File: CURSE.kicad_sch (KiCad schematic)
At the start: 25 parts, among them J1 USB_C_Receptacle_USB2.0_14P, U1 RP2040, U2 NCP1117-3.3_SOT223, Y1 12 Mhz

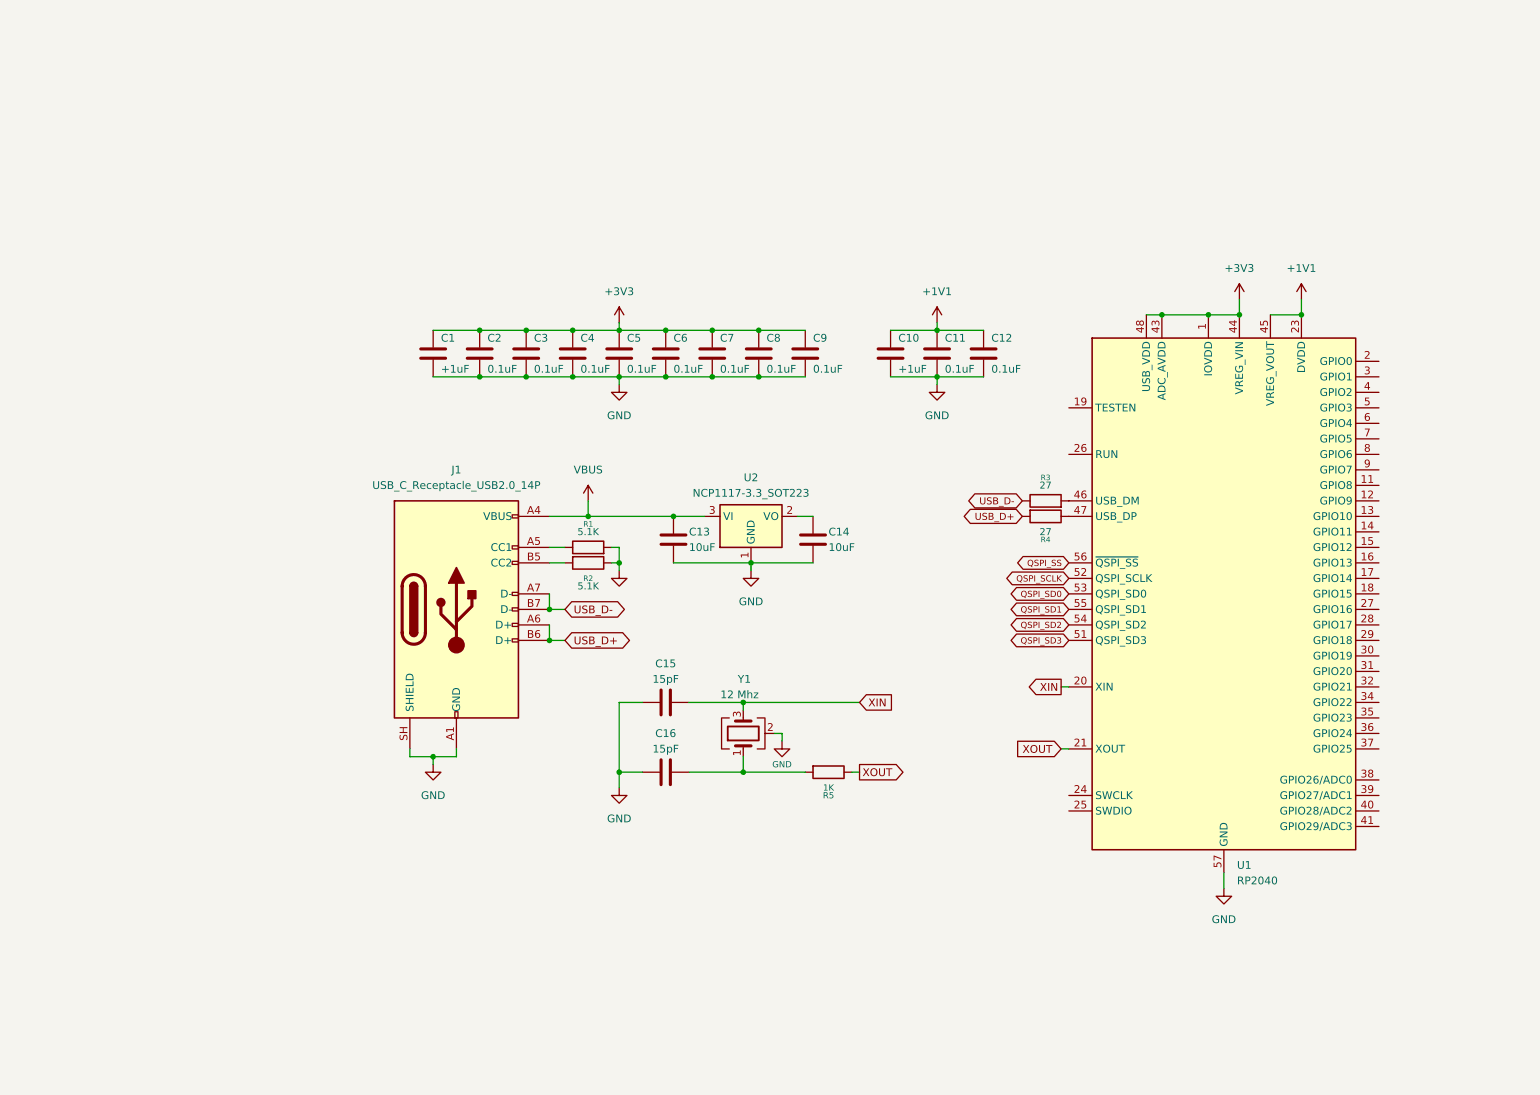
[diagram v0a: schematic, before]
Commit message: now going on with pcb!! check the devlog for what made
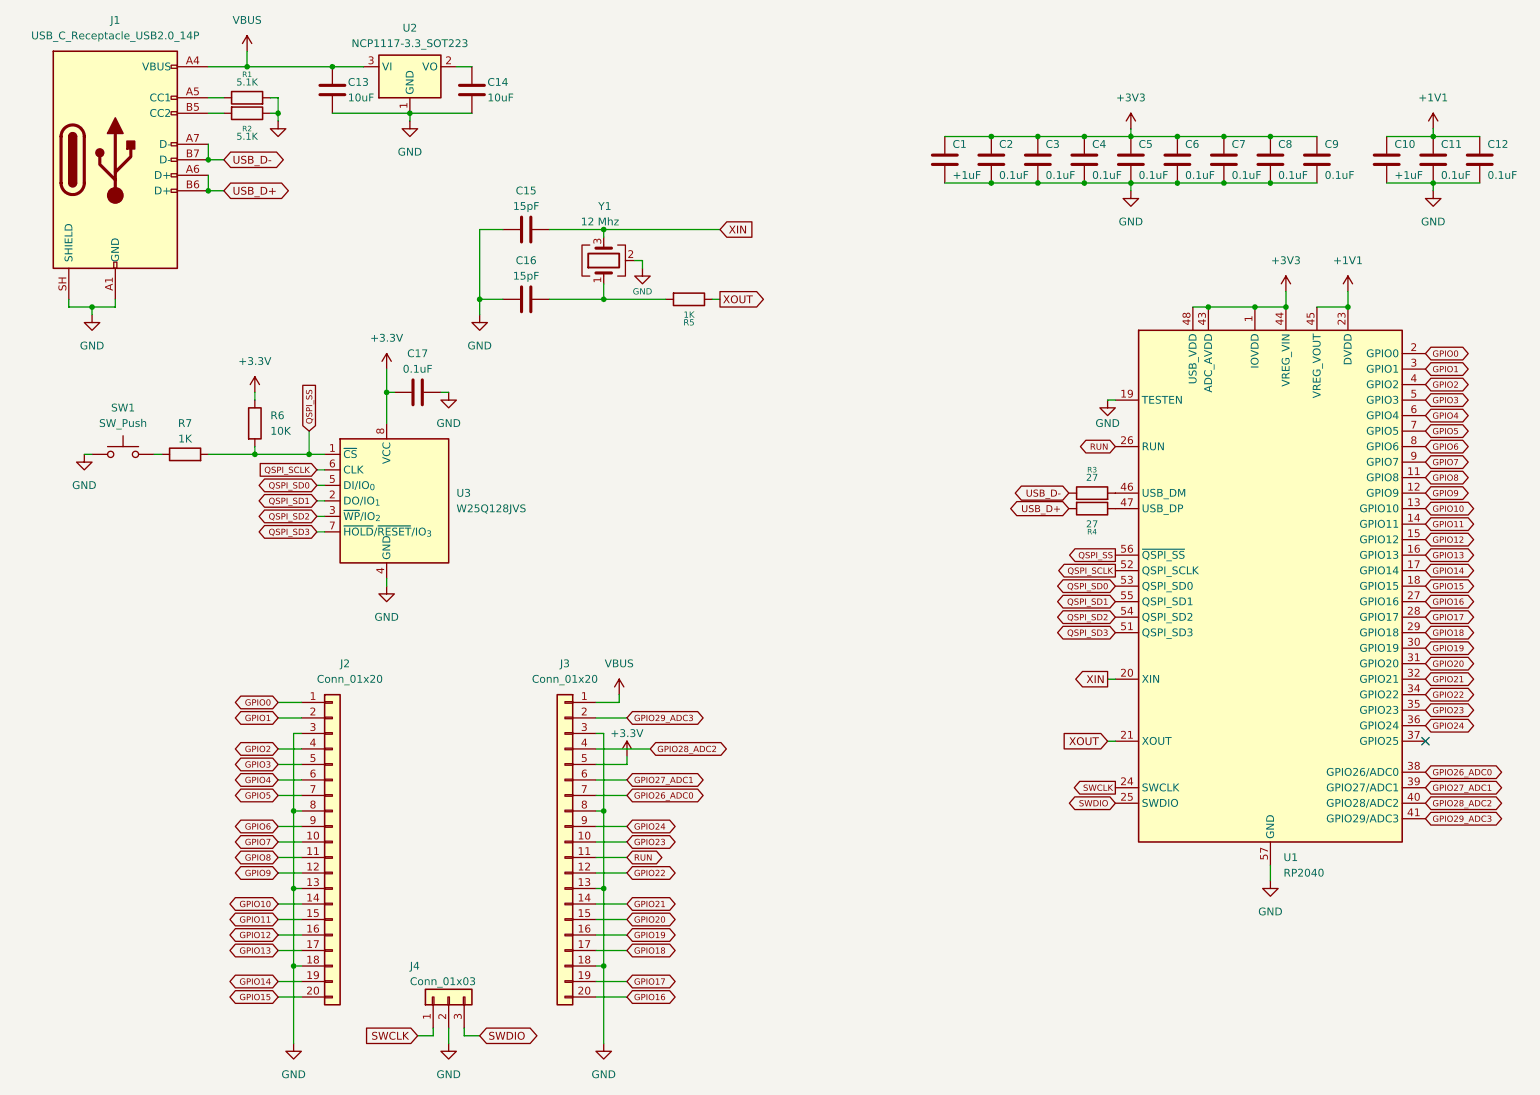
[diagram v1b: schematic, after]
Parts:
- added C17: 0.1uF, symbol Device:C
- added J2, J3: Conn_01x20, symbol Connector_Generic:Conn_01x20
- added J4: Conn_01x03, symbol Connector_Generic:Conn_01x03
- added R6: 10K, symbol Device:R
- added R7: 1K, symbol Device:R
- added SW1: SW_Push, symbol Switch:SW_Push
- added U3: W25Q128JVS, Package_SO:SOIC-8_5.3x5.3mm_P1.27mm, symbol Memory_Flash:W25Q128JVS
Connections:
- net GND: now also U1.19 (TESTEN), C17.2, J2.13 (Pin_13), J2.18 (Pin_18), J2.3 (Pin_3), J2.8 (Pin_8), J3.13 (Pin_13), J3.18 (Pin_18), J3.3 (Pin_3), J3.8 (Pin_8), J4.2 (Pin_2), SW1.1, U3.4 (GND)
- net QSPI_SCLK: now also U3.6 (CLK)
- net QSPI_SD0: now also U3.5 (DI/IO_{0})
- net QSPI_SD1: now also U3.2 (DO/IO_{1})
- net QSPI_SD2: now also U3.3 (~{WP}/IO_{2})
- net QSPI_SD3: now also U3.7 (~{HOLD}/~{RESET}/IO_{3})
- net QSPI_SS: now also R6.2, R7.2, U3.1 (~{CS})
- net VBUS: now also J3.1 (Pin_1)
- net GPIO8: now reaches U1.11 (GPIO8)
- net GPIO8: now also J2.11 (Pin_11)
- net GPIO9: now reaches U1.12 (GPIO9)
- net GPIO9: now also J2.12 (Pin_12)
- net GPIO10: now reaches U1.13 (GPIO10)
- net GPIO10: now also J2.14 (Pin_14)
- net GPIO11: now reaches U1.14 (GPIO11)
- net GPIO11: now also J2.15 (Pin_15)
- net GPIO12: now reaches U1.15 (GPIO12)
- net GPIO12: now also J2.16 (Pin_16)
- net GPIO13: now reaches U1.16 (GPIO13)
- net GPIO13: now also J2.17 (Pin_17)
- net GPIO14: now reaches U1.17 (GPIO14)
- net GPIO14: now also J2.19 (Pin_19)
- net GPIO15: now reaches U1.18 (GPIO15)
- net GPIO15: now also J2.20 (Pin_20)
- net GPIO0: now reaches U1.2 (GPIO0)
- net GPIO0: now also J2.1 (Pin_1)
- net SWCLK: now reaches U1.24 (SWCLK)
- net SWCLK: now also J4.1 (Pin_1)
- net SWDIO: now reaches U1.25 (SWDIO)
- net SWDIO: now also J4.3 (Pin_3)
- net RUN: now reaches U1.26 (RUN)
- net RUN: now also J3.11 (Pin_11)
- net GPIO16: now reaches U1.27 (GPIO16)
- net GPIO16: now also J3.20 (Pin_20)
- net GPIO17: now reaches U1.28 (GPIO17)
- net GPIO17: now also J3.19 (Pin_19)
- net GPIO18: now reaches U1.29 (GPIO18)
- net GPIO18: now also J3.17 (Pin_17)
- net GPIO1: now reaches U1.3 (GPIO1)
- net GPIO1: now also J2.2 (Pin_2)
- net GPIO19: now reaches U1.30 (GPIO19)
- net GPIO19: now also J3.16 (Pin_16)
- net GPIO20: now reaches U1.31 (GPIO20)
- net GPIO20: now also J3.15 (Pin_15)
- net GPIO21: now reaches U1.32 (GPIO21)
- net GPIO21: now also J3.14 (Pin_14)
- net GPIO22: now reaches U1.34 (GPIO22)
- net GPIO22: now also J3.12 (Pin_12)
- net GPIO23: now reaches U1.35 (GPIO23)
- net GPIO23: now also J3.10 (Pin_10)
- net GPIO24: now reaches U1.36 (GPIO24)
- net GPIO24: now also J3.9 (Pin_9)
- net GPIO26_ADC0: now reaches U1.38 (GPIO26/ADC0)
- net GPIO26_ADC0: now also J3.7 (Pin_7)
- net GPIO27_ADC1: now reaches U1.39 (GPIO27/ADC1)
- net GPIO27_ADC1: now also J3.6 (Pin_6)
- net GPIO2: now reaches U1.4 (GPIO2)
- net GPIO2: now also J2.4 (Pin_4)
- net GPIO28_ADC2: now reaches U1.40 (GPIO28/ADC2)
- net GPIO28_ADC2: now also J3.4 (Pin_4)
- net GPIO29_ADC3: now reaches U1.41 (GPIO29/ADC3)
- net GPIO29_ADC3: now also J3.2 (Pin_2)
- net GPIO3: now reaches U1.5 (GPIO3)
- net GPIO3: now also J2.5 (Pin_5)
- net GPIO4: now reaches U1.6 (GPIO4)
- net GPIO4: now also J2.6 (Pin_6)
- net GPIO5: now reaches U1.7 (GPIO5)
- net GPIO5: now also J2.7 (Pin_7)
- net GPIO6: now reaches U1.8 (GPIO6)
- net GPIO6: now also J2.9 (Pin_9)
- net GPIO7: now reaches U1.9 (GPIO7)
- net GPIO7: now also J2.10 (Pin_10)
- new net: R7.1, SW1.2
- new net +3.3V: C17.1, J3.5 (Pin_5), R6.1, U3.8 (VCC)
- no-connect marks 0 -> 1
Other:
- moved on the sheet: C1, C10, C11, C12, C13, C14, C15, C16, C2, C3, C4, C5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

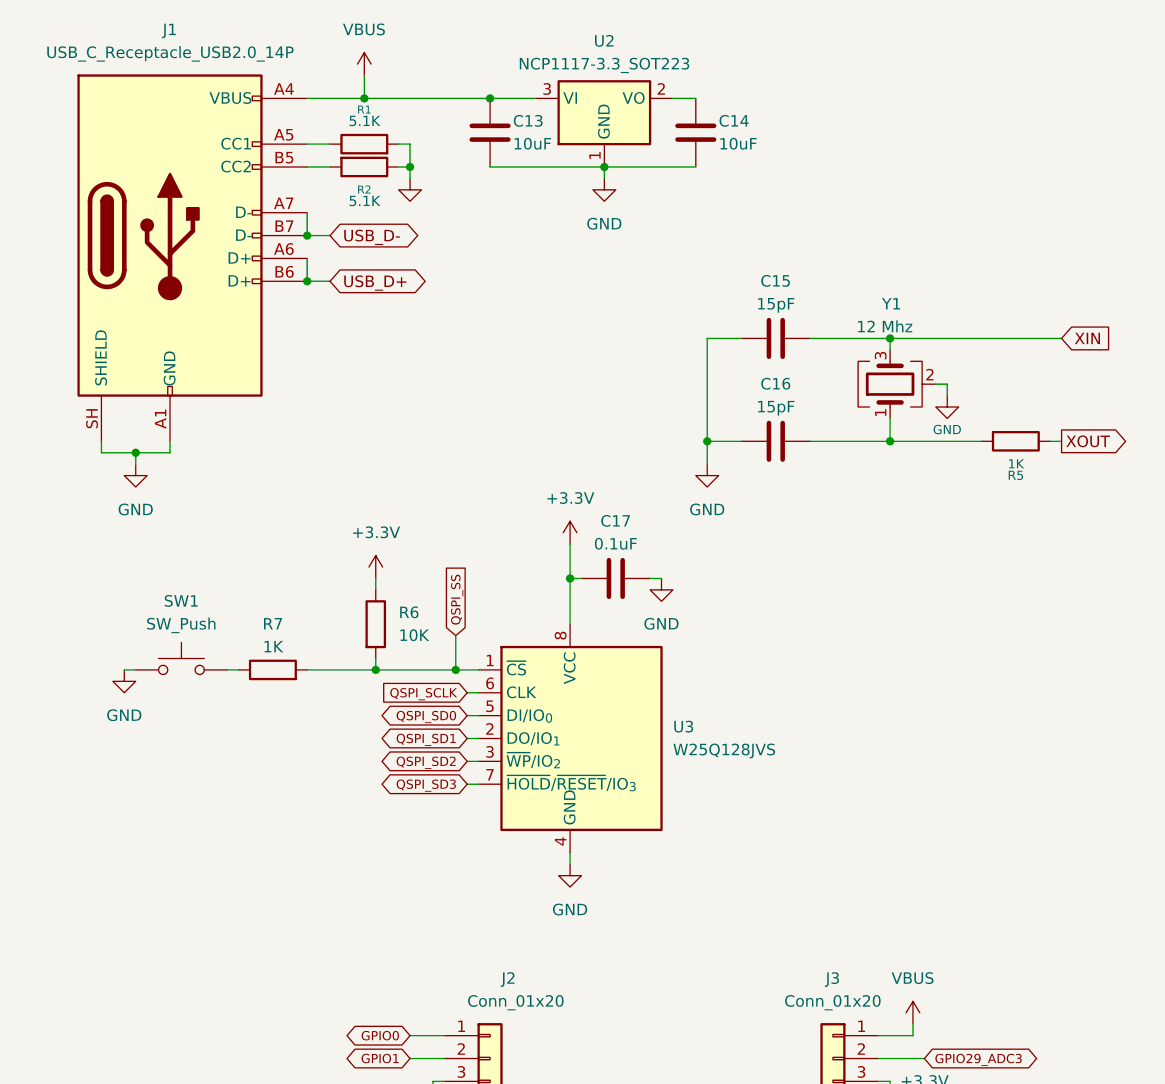
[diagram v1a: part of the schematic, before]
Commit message: check the journal bro im just pushing
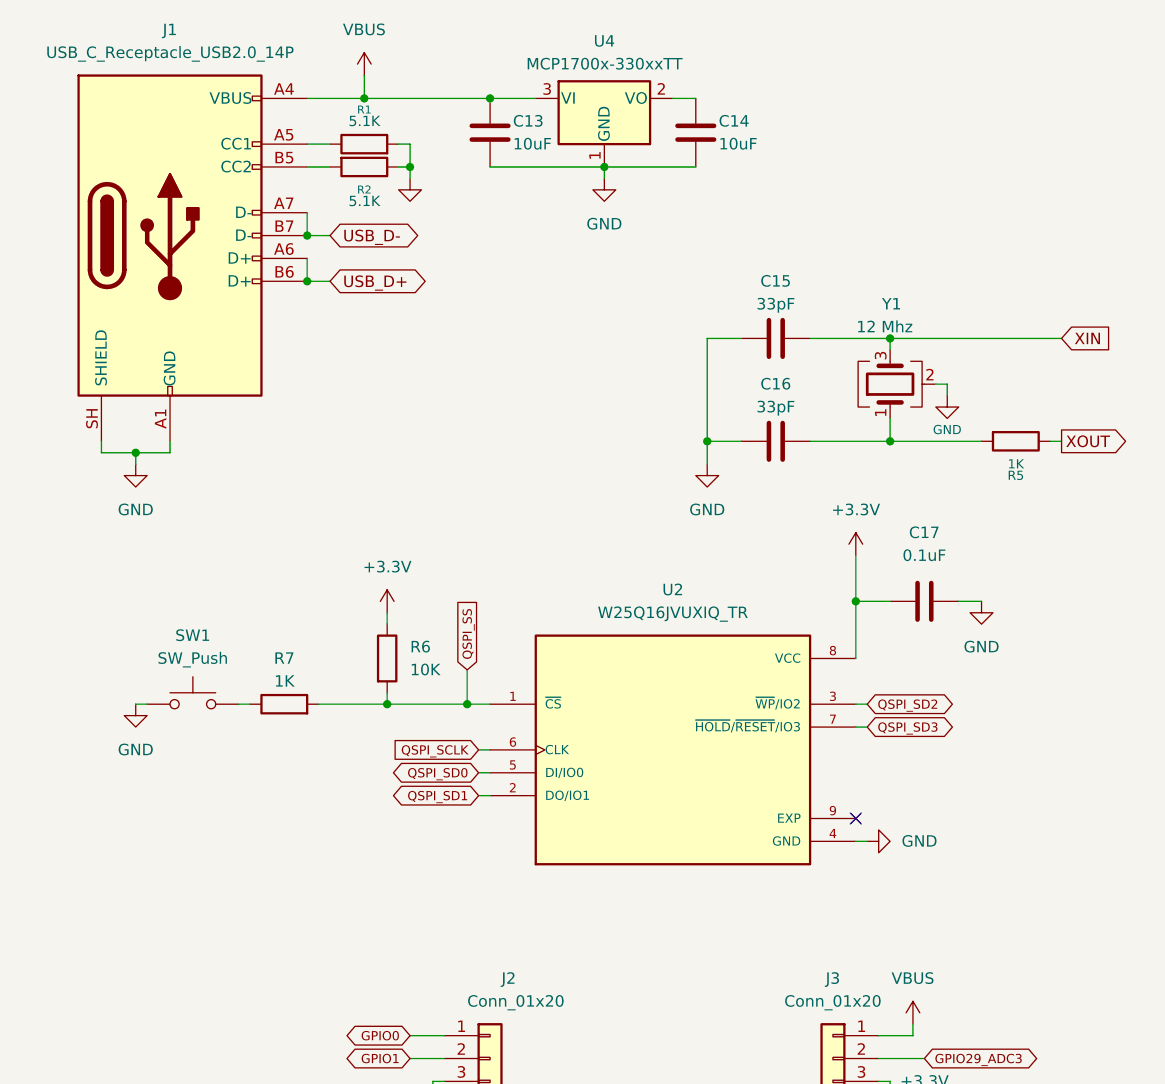
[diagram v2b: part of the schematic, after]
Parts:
- removed U2: NCP1117-3.3_SOT223, Package_TO_SOT_SMD:SOT-223-3_TabPin2, symbol Regulator_Linear:NCP1117-3.3_SOT223
- removed U3: W25Q128JVS, Package_SO:SOIC-8_5.3x5.3mm_P1.27mm, symbol Memory_Flash:W25Q128JVS
- added U2: W25Q16JVUXIQ_TR, Package_SON:Winbond_USON-8-1EP_3x2mm_P0.5mm_EP0.2x1.6mm, symbol W25Q16JVUXIQ_TR:W25Q16JVUXIQ_TR
- added U4: MCP1700x-330xxTT, Package_TO_SOT_SMD:SOT-23, symbol Regulator_Linear:MCP1700x-330xxTT
- C1, C10, C11, C12, C17, C2, C3, C4, C5, C6, C7, C8, C9: footprint (none) -> Capacitor_SMD:C_0402_1005Metric
- C13, C14: footprint (none) -> Capacitor_SMD:C_0603_1608Metric
- C15, C16: value 15pF -> 33pF; footprint (none) -> Capacitor_SMD:C_0402_1005Metric
- J1: footprint (none) -> Connector_USB:USB_C_Receptacle_HRO_TYPE-C-31-M-12
- J2, J3: footprint (none) -> Connector_PinHeader_2.54mm:PinHeader_1x20_P2.54mm_Vertical
- J4: footprint (none) -> Connector_PinHeader_2.54mm:PinHeader_1x03_P2.54mm_Vertical
- R1, R2, R3, R4, R5, R6, R7: footprint (none) -> Resistor_SMD:R_0402_1005Metric
- SW1: footprint (none) -> Button_Switch_SMD:SW_Push_SPST_NO_Alps_SKRK
- Y1: footprint Crystal:Crystal_SMD_0603-4Pin_6.0x3.5mm -> Crystal:Crystal_SMD_3225-4Pin_3.2x2.5mm
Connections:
- net +3.3V: now also U2.8 (VCC)
- net GND: now also U2.4 (GND), U4.1 (GND)
- net QSPI_SCLK: now also U2.6 (CLK)
- net QSPI_SD0: now also U2.5 (DI/IO0)
- net QSPI_SD1: now also U2.2 (DO/IO1)
- net QSPI_SD2: now also U2.3 (~{WP}/IO2)
- net QSPI_SD3: now also U2.7 (~{HOLD}/~{RESET}/IO3)
- net QSPI_SS: now also U2.1 (~{CS})
- net VBUS: now also U4.3 (VI)
- net at C14.1: now also U4.2 (VO)
- no-connect marks 1 -> 2
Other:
- moved on the sheet: R6, R7, SW1
